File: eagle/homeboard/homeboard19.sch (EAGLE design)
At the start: 136 parts, among them IC1 XCF02S, IC2 25LC080SN, IC3 ATMEGA32U2-TQFP, Q5 BC848SMD, Q6 BC848SMD, Q7 BC848SMD, Q8 BC848SMD, T1 BSS138, T2 BC848, T3 BSS138, T4 BC848, U1 XC3S400TQ144, X1 SCART-CLIP, X6 MINI-USB_4P-85-32004-10X, X7 DC21MMX, X8 STEREOJACK

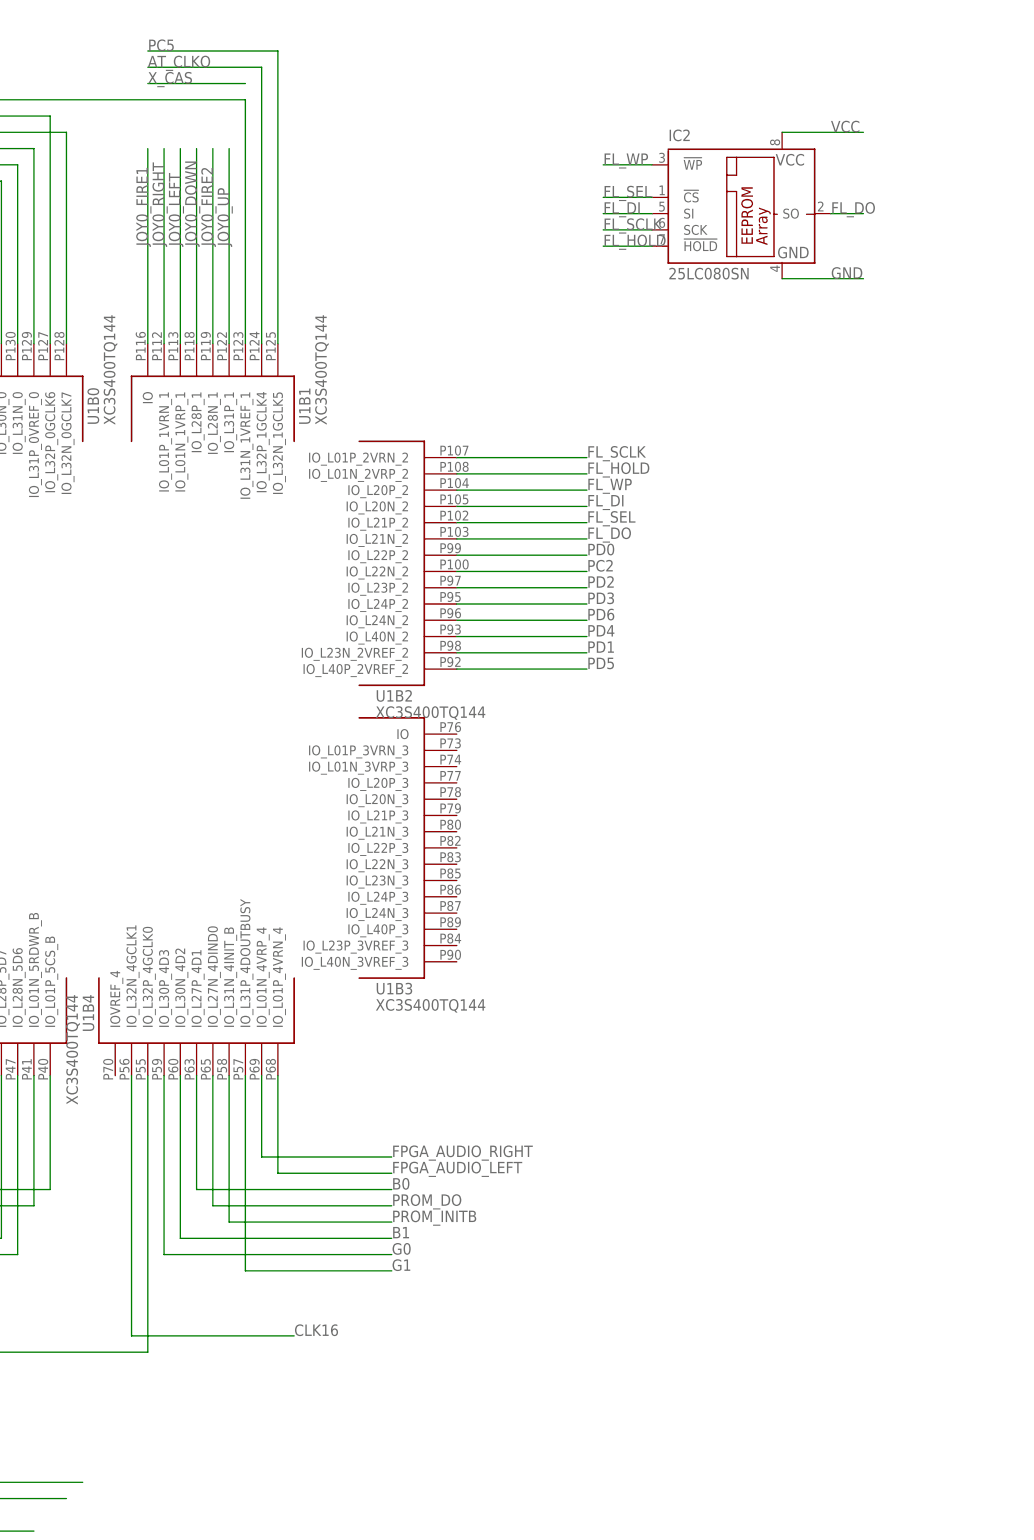
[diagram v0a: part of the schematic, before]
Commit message: mah
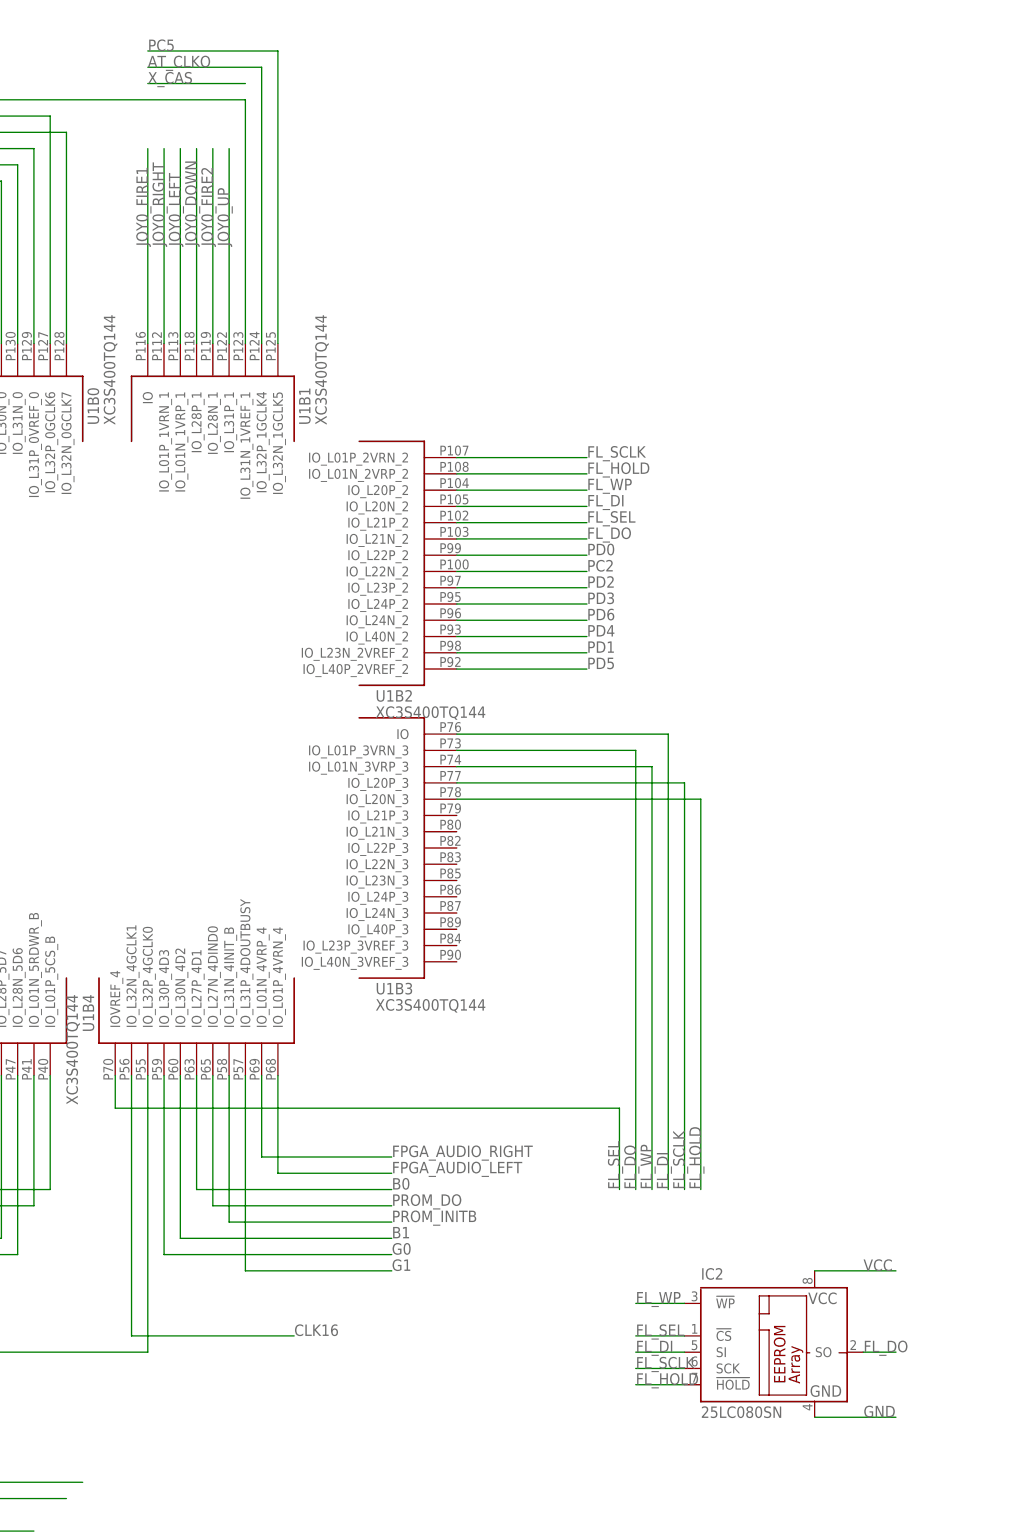
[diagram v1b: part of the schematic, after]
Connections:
- net FL_DI: now also U1B3.IO
- net FL_DO: now also U1B3.IO_L01P_3VRN_3
- net FL_HOLD: now also U1B3.IO_L20N_3
- net FL_SCLK: now also U1B3.IO_L20P_3
- net FL_SEL: now also U1B4.IOVREF_4
- net FL_WP: now also U1B3.IO_L01N_3VRP_3
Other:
- moved on the sheet: IC2
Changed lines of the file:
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@@
 <instance part="SUPPLY4" gate="GND" x="-20.32" y="152.4"/>
 <instance part="SUPPLY5" gate="GND" x="-20.32" y="198.12"/>
-<instance part="IC2" gate="G$1" x="254" y="93.98"/>
+<instance part="IC2" gate="G$1" x="259.08" y="-83.82"/>
 <instance part="R48" gate="G$1" x="144.78" y="177.8"/>
 <instance part="C1" gate="G$1" x="132.08" y="172.72" rot="R180"/>
@@
 <segment>
 <pinref part="IC2" gate="G$1" pin="GND"/>
-<wire x1="274.32" y1="83.82" x2="261.62" y2="83.82" width="0.1524" layer="91"/>
-<label x="269.24" y="83.82" size="1.778" layer="95"/>
+<wire x1="279.4" y1="-93.98" x2="266.7" y2="-93.98" width="0.1524" layer="91"/>
+<label x="274.32" y="-93.98" size="1.778" layer="95"/>
 </segment>
 <segment>
@@
 <segment>
 <pinref part="IC2" gate="G$1" pin="VCC"/>
-<label x="269.24" y="106.68" size="1.778" layer="95"/>
-<wire x1="261.62" y1="106.68" x2="274.32" y2="106.68" width="0.1524" layer="91"/>
+<label x="274.32" y="-71.12" size="1.778" layer="95"/>
+<wire x1="266.7" y1="-71.12" x2="279.4" y2="-71.12" width="0.1524" layer="91"/>
 </segment>
 <segment>
@@
 <segment>
 <pinref part="IC2" gate="G$1" pin="!CS"/>
-<wire x1="233.68" y1="96.52" x2="241.3" y2="96.52" width="0.1524" layer="91"/>
-<label x="233.68" y="96.52" size="1.778" layer="95"/>
+<wire x1="238.76" y1="-81.28" x2="246.38" y2="-81.28" width="0.1524" layer="91"/>
+<label x="238.76" y="-81.28" size="1.778" layer="95"/>
 </segment>
 <segment>
@@
 <wire x1="231.14" y1="45.72" x2="210.82" y2="45.72" width="0.1524" layer="91"/>
 <label x="231.14" y="45.72" size="1.778" layer="95"/>
+</segment>
+<segment>
+<pinref part="U1" gate="B4" pin="IOVREF_4"/>
+<wire x1="236.22" y1="-45.72" x2="157.48" y2="-45.72" width="0.1524" layer="91"/>
+<wire x1="157.48" y1="-45.72" x2="157.48" y2="-40.64" width="0.1524" layer="91"/>
+<wire x1="236.22" y1="-58.42" x2="236.22" y2="-45.72" width="0.1524" layer="91"/>
+<label x="236.22" y="-58.42" size="1.778" layer="95" rot="R90"/>
 </segment>
 </net>
@@
 <segment>
 <pinref part="IC2" gate="G$1" pin="!HOLD"/>
-<label x="233.68" y="88.9" size="1.778" layer="95"/>
-<wire x1="233.68" y1="88.9" x2="241.3" y2="88.9" width="0.1524" layer="91"/>
+<label x="238.76" y="-88.9" size="1.778" layer="95"/>
+<wire x1="238.76" y1="-88.9" x2="246.38" y2="-88.9" width="0.1524" layer="91"/>
 </segment>
 <segment>
@@
 <label x="231.14" y="53.34" size="1.778" layer="95"/>
 </segment>
+<segment>
+<pinref part="U1" gate="B3" pin="IO_L20N_3"/>
+<wire x1="210.82" y1="2.54" x2="248.92" y2="2.54" width="0.1524" layer="91"/>
+<wire x1="248.92" y1="2.54" x2="248.92" y2="-58.42" width="0.1524" layer="91"/>
+<label x="248.92" y="-58.42" size="1.778" layer="95" rot="R90"/>
+</segment>
 </net>
 <net name="FL_SCLK" class="0">
 <segment>
 <pinref part="IC2" gate="G$1" pin="SCK"/>
-<wire x1="233.68" y1="91.44" x2="241.3" y2="91.44" width="0.1524" layer="91"/>
-<label x="233.68" y="91.44" size="1.778" layer="95"/>
+<wire x1="238.76" y1="-86.36" x2="246.38" y2="-86.36" width="0.1524" layer="91"/>
+<label x="238.76" y="-86.36" size="1.778" layer="95"/>
 </segment>
 <segment>
@@
 <label x="231.14" y="55.88" size="1.778" layer="95"/>
 </segment>
+<segment>
+<pinref part="U1" gate="B3" pin="IO_L20P_3"/>
+<wire x1="210.82" y1="5.08" x2="246.38" y2="5.08" width="0.1524" layer="91"/>
+<wire x1="246.38" y1="5.08" x2="246.38" y2="-58.42" width="0.1524" layer="91"/>
+<label x="246.38" y="-58.42" size="1.778" layer="95" rot="R90"/>
+</segment>
 </net>
 <net name="FL_DI" class="0">
 <segment>
 <pinref part="IC2" gate="G$1" pin="SI"/>
-<wire x1="233.68" y1="93.98" x2="241.3" y2="93.98" width="0.1524" layer="91"/>
-<label x="233.68" y="93.98" size="1.778" layer="95"/>
+<wire x1="238.76" y1="-83.82" x2="246.38" y2="-83.82" width="0.1524" layer="91"/>
+<label x="238.76" y="-83.82" size="1.778" layer="95"/>
 </segment>
 <segment>
@@
 <label x="231.14" y="48.26" size="1.778" layer="95"/>
 </segment>
+<segment>
+<wire x1="243.84" y1="-58.42" x2="243.84" y2="12.7" width="0.1524" layer="91"/>
+<pinref part="U1" gate="B3" pin="IO"/>
+<wire x1="243.84" y1="12.7" x2="210.82" y2="12.7" width="0.1524" layer="91"/>
+<label x="243.84" y="-58.42" size="1.778" layer="95" rot="R90"/>
+</segment>
 </net>
 <net name="FL_DO" class="0">
 <segment>
 <pinref part="IC2" gate="G$1" pin="SO"/>
-<wire x1="274.32" y1="93.98" x2="269.24" y2="93.98" width="0.1524" layer="91"/>
-<label x="269.24" y="93.98" size="1.778" layer="95"/>
+<wire x1="279.4" y1="-83.82" x2="274.32" y2="-83.82" width="0.1524" layer="91"/>
+<label x="274.32" y="-83.82" size="1.778" layer="95"/>
 </segment>
 <segment>
@@
 <label x="231.14" y="43.18" size="1.778" layer="95"/>
 </segment>
+<segment>
+<wire x1="238.76" y1="-58.42" x2="238.76" y2="10.16" width="0.1524" layer="91"/>
+<pinref part="U1" gate="B3" pin="IO_L01P_3VRN_3"/>
+<wire x1="238.76" y1="10.16" x2="210.82" y2="10.16" width="0.1524" layer="91"/>
+<label x="238.76" y="-58.42" size="1.778" layer="95" rot="R90"/>
+</segment>
 </net>
 <net name="FL_WP" class="0">
 <segment>
 <pinref part="IC2" gate="G$1" pin="!WP"/>
-<wire x1="233.68" y1="101.6" x2="241.3" y2="101.6" width="0.1524" layer="91"/>
-<label x="233.68" y="101.6" size="1.778" layer="95"/>
+<wire x1="238.76" y1="-76.2" x2="246.38" y2="-76.2" width="0.1524" layer="91"/>
+<label x="238.76" y="-76.2" size="1.778" layer="95"/>
 </segment>
 <segment>
@@
 <label x="231.14" y="50.8" size="1.778" layer="95"/>
 </segment>
-</net>
+<segment>
+<pinref part="U1" gate="B3" pin="IO_L01N_3VRP_3"/>
+<wire x1="210.82" y1="7.62" x2="241.3" y2="7.62" width="0.1524" layer="91"/>
+<wire x1="241.3" y1="7.62" x2="241.3" y2="-58.42" width="0.1524" layer="91"/>
+<label x="241.3" y="-58.42" size="1.778" layer="95" rot="R90"/>
+</segment>
+</net>
